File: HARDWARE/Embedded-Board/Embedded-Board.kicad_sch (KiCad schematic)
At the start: 5 parts, among them J1 SENSOR SOCKET, J2 POWER-pins, J3 Conn_02x20_Odd_Even, SW1 SW_Push, SW2 RotaryEncoder_Switch

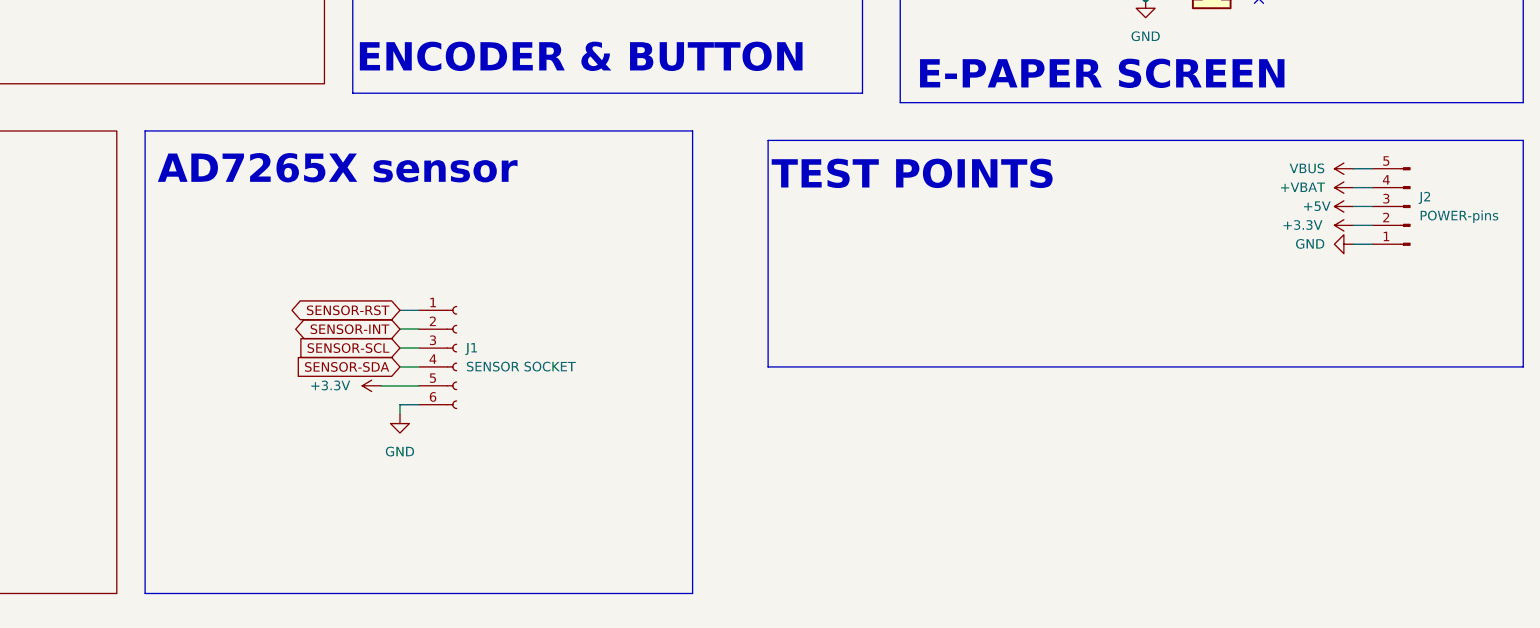
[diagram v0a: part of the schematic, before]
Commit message: New PCB design for JLCPCB
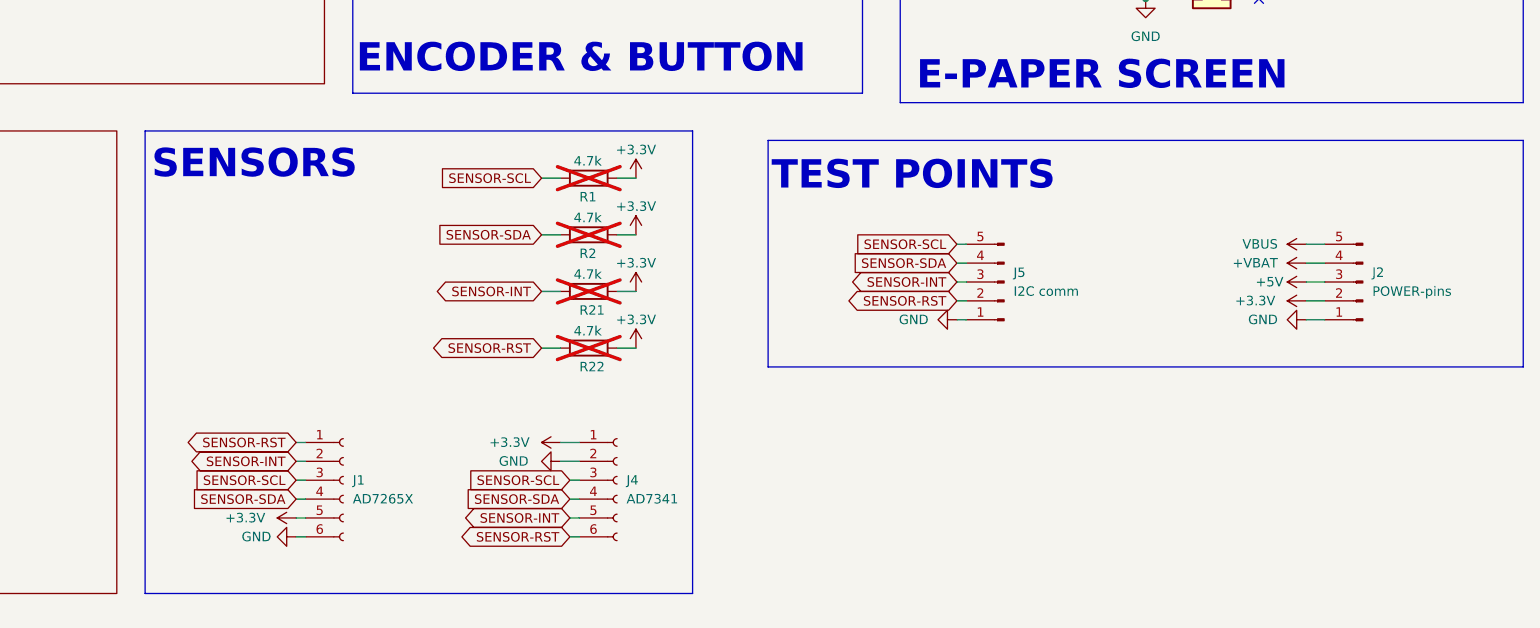
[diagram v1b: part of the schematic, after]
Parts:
- added J4: AD7341, Connector_PinSocket_2.54mm:PinSocket_1x06_P2.54mm_Vertical, symbol Connector:Conn_01x06_Socket
- added J5: I2C comm, Connector_PinHeader_2.54mm:PinHeader_1x05_P2.54mm_Vertical, symbol Connector:Conn_01x05_Pin
- added R1, R2, R21, R22: 4.7k, Resistor_SMD:R_0805_2012Metric, symbol Device:R
- J1: value SENSOR SOCKET -> AD7265X; footprint (none) -> Connector_PinSocket_2.54mm:PinSocket_1x06_P2.54mm_Vertical
- J2: footprint (none) -> Connector_PinHeader_2.54mm:PinHeader_1x05_P2.54mm_Vertical
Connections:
- net +3.3V: now also J4.1 (Pin_1), R1.1, R2.1, R21.1, R22.1
- net GND: now also J4.2 (Pin_2), J5.1 (Pin_1)
- net SENSOR-INT: now also J4.5 (Pin_5), J5.3 (Pin_3), R21.2
- net SENSOR-RST: now also J4.6 (Pin_6), J5.2 (Pin_2), R22.2
- net SENSOR-SCL: now also J4.3 (Pin_3), J5.5 (Pin_5), R1.2
- net SENSOR-SDA: now also J4.4 (Pin_4), J5.4 (Pin_4), R2.2
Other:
- note added: "SENSORS"
- note removed: "AD7265X sensor"
- title: Low Cost VIS/NIF Spectrometer -> Low Cost VIS/NIR Spectrometer
- moved on the sheet: J1, J2

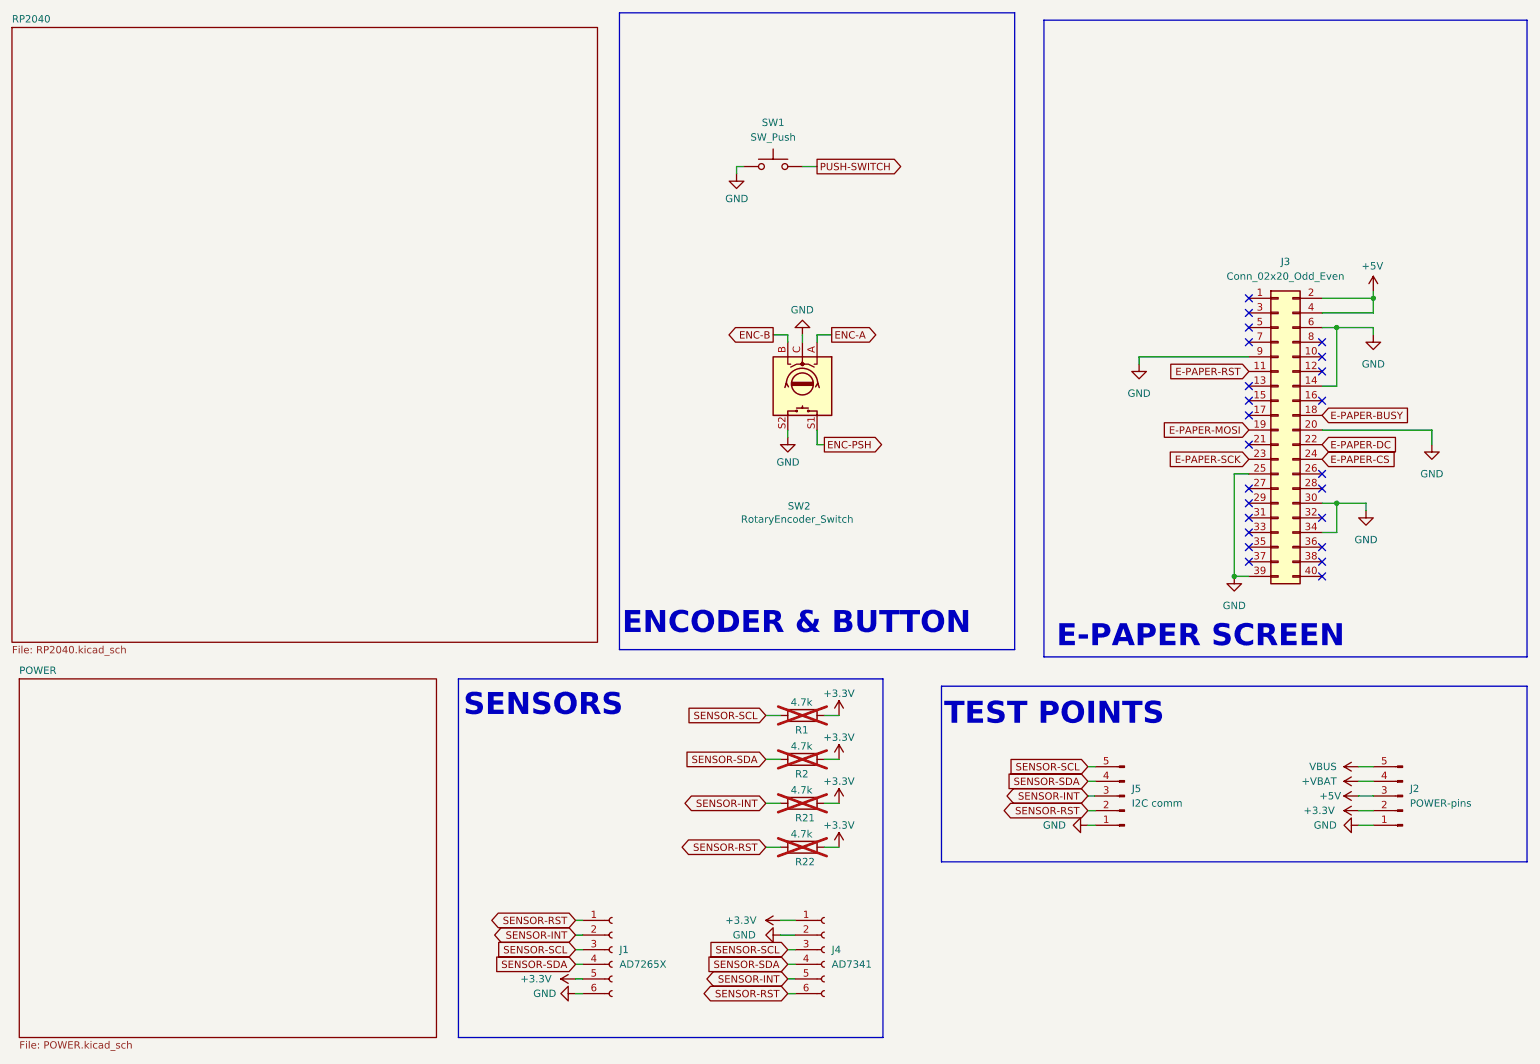
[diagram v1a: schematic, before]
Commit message: Final PCB version
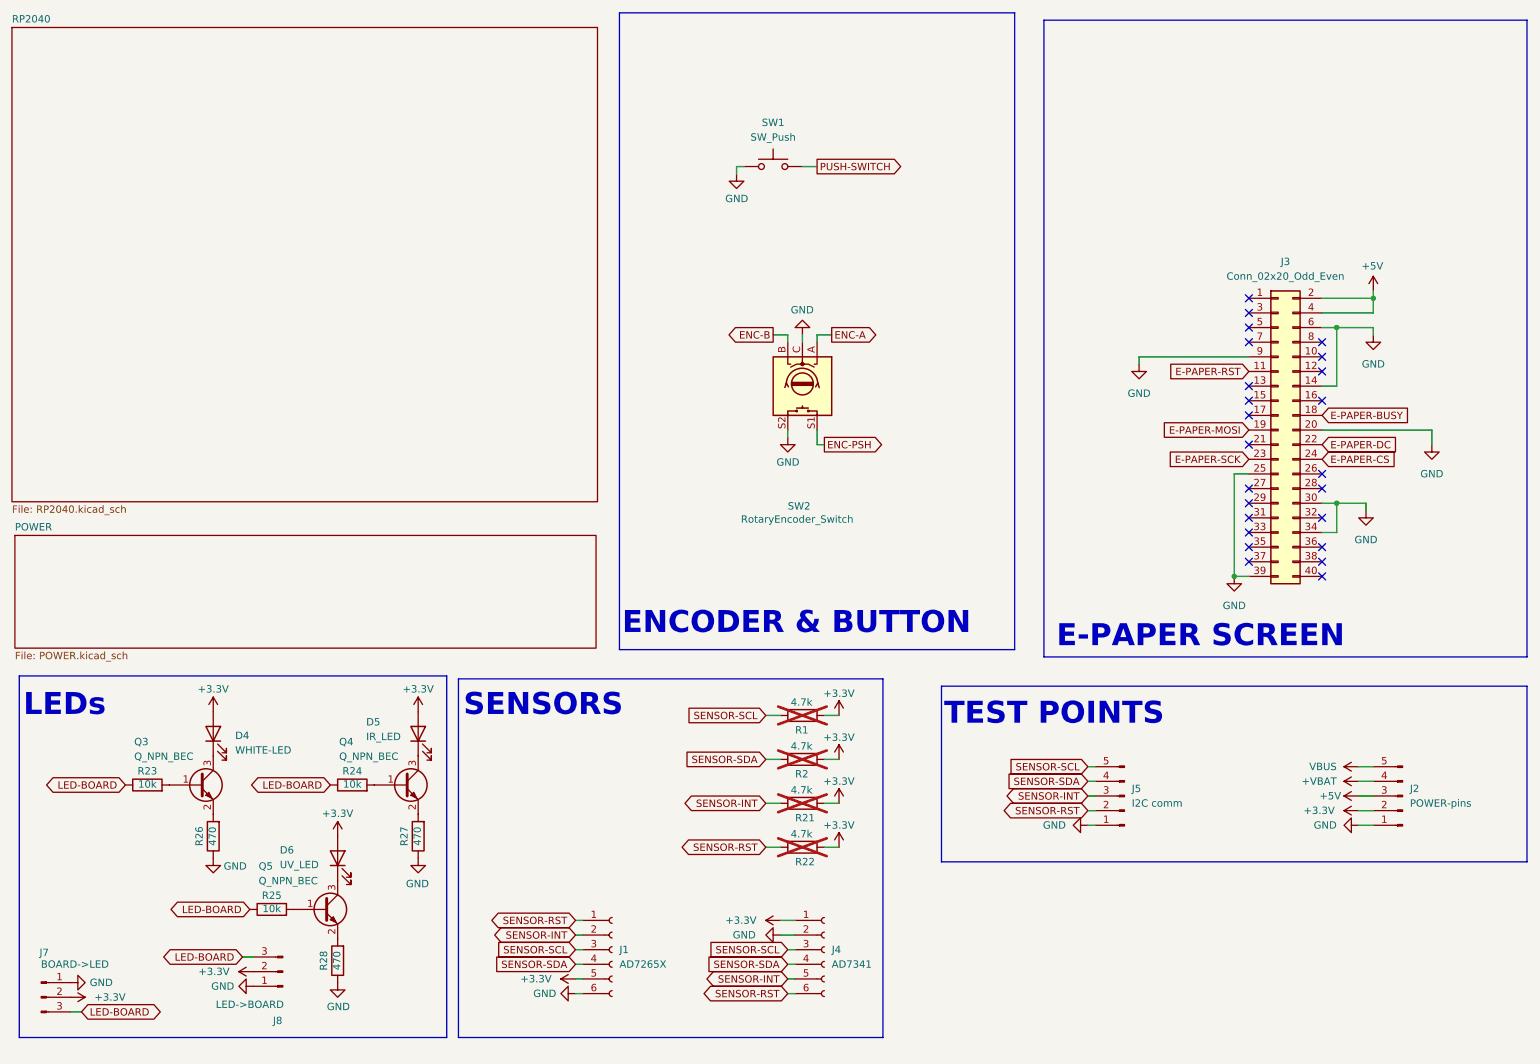
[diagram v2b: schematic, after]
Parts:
- added D4: WHITE-LED, LED_SMD:LED_1206_3216Metric, symbol Device:LED
- added D5: IR_LED, LED_SMD:LED_0805_2012Metric, symbol Device:LED
- added D6: UV_LED, LED_SMD:LED_PLCC_2835, symbol Device:LED
- added J7: BOARD->LED, Connector_PinHeader_2.54mm:PinHeader_1x03_P2.54mm_Vertical, symbol Connector:Conn_01x03_Pin
- added J8: LED->BOARD, Connector_PinHeader_2.54mm:PinHeader_1x03_P2.54mm_Vertical, symbol Connector:Conn_01x03_Pin
- added Q3, Q4, Q5: Q_NPN_BEC, Package_TO_SOT_THT:TO-92_Wide, symbol Device:Q_NPN_BEC
- added R23, R24, R25: 10k, Resistor_THT:R_Axial_DIN0411_L9.9mm_D3.6mm_P12.70mm_Horizontal, symbol Device:R
- added R26, R27, R28: 470, Resistor_THT:R_Axial_DIN0411_L9.9mm_D3.6mm_P12.70mm_Horizontal, symbol Device:R
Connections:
- net +3.3V: now also D4.2 (A), D5.2 (A), D6.2 (A), J7.2 (Pin_2), J8.2 (Pin_2)
- net GND: now also J7.1 (Pin_1), J8.1 (Pin_1), R26.1, R27.1, R28.1
- new net: Q3.1 (B), R23.2
- new net: Q3.2 (E), R26.2
- new net: D4.1 (K), Q3.3 (C)
- new net: Q4.1 (B), R24.2
- new net: Q5.1 (B), R25.2
- new net: Q5.2 (E), R28.2
- new net: D6.1 (K), Q5.3 (C)
- new net: D5.1 (K), Q4.3 (C)
- new net: Q4.2 (E), R27.2
- new net LED-BOARD: J7.3 (Pin_3), J8.3 (Pin_3), R23.1, R24.1, R25.1
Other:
- note added: "LEDs"
